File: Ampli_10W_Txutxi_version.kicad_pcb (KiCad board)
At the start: 2 copper layers, 35.3 x 31.7 mm, 9 parts, among them U1 TDA2003V

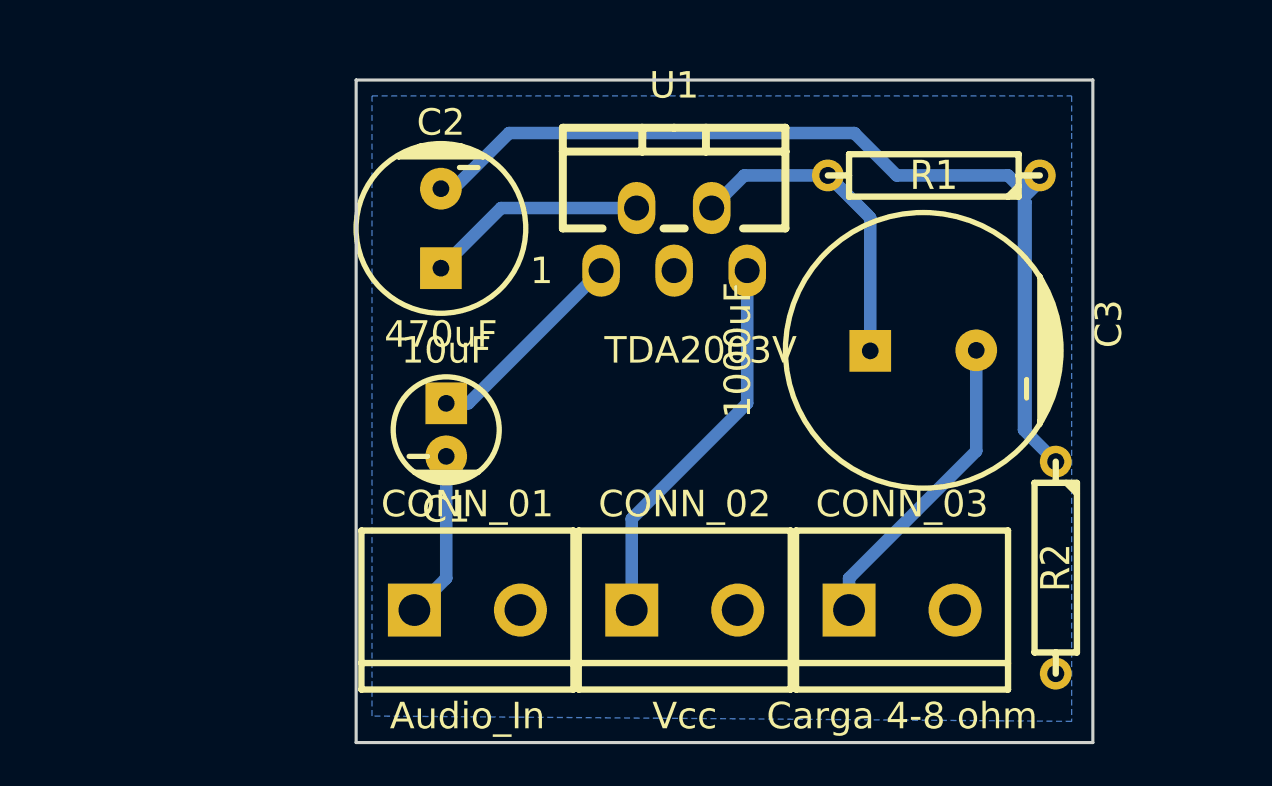
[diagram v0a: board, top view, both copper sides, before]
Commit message: Update library and PCB
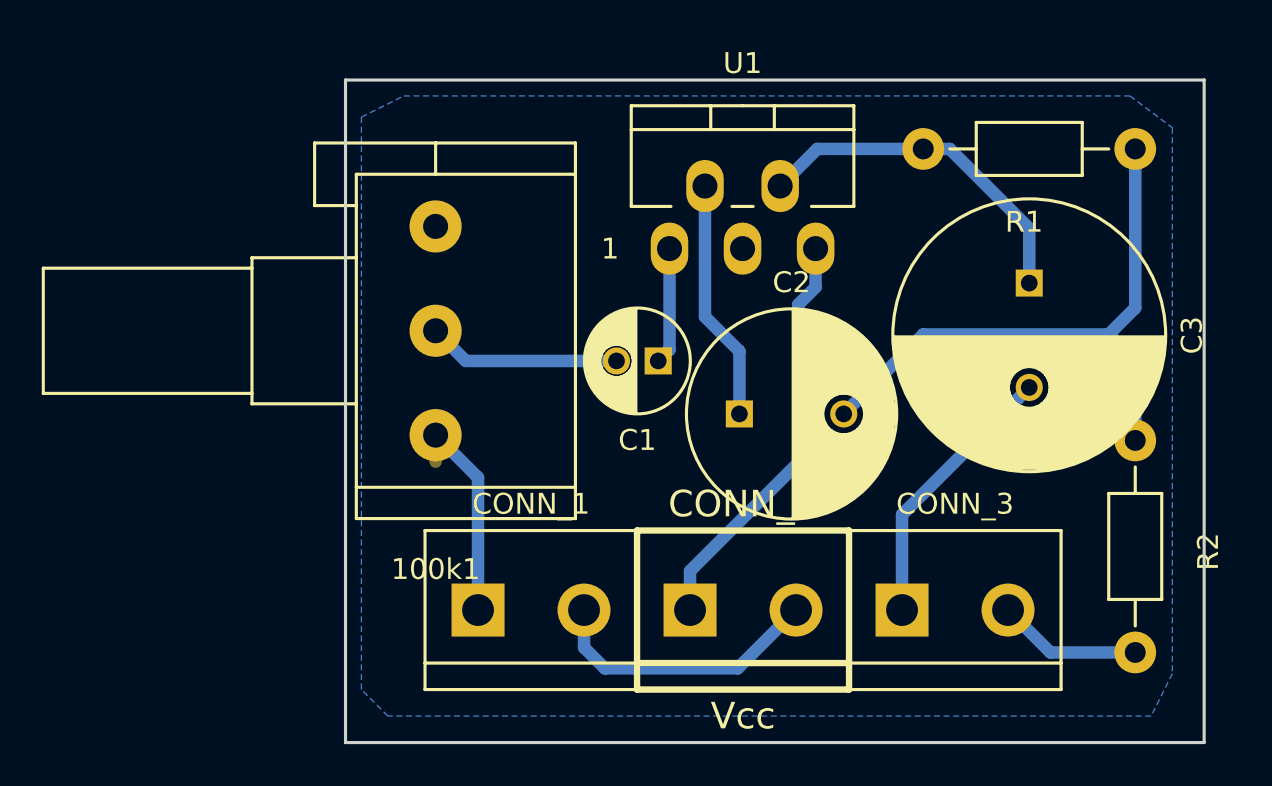
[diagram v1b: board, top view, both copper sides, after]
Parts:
- removed CONN_01: Audio_In, Connect:bornier2
- removed CONN_03: Carga 4-8 ohm, Connect:bornier2
- added 100k1: POT, Potentiometers:Potentiometer_Alps-RK16-single, F.Cu at (140.5, 114.0)
- added CONN_1: Audio_In, Connect:bornier2, F.Cu at (145.0, 122.4)
- added CONN_3: Carga 4-8 ohm, Connect:bornier2, F.Cu at (165.4, 122.4)
- C1: footprint Capacitors:CP_5x11mm -> Capacitors_ThroughHole:C_Radial_D5_L11_P2
- C2: footprint Capacitors:CP_8x21mm -> Capacitors_ThroughHole:C_Radial_D10_L16_P5
- C3: footprint Capacitors:CP_13x21mm -> Capacitors_ThroughHole:C_Radial_D13_L21_P5
- R1, R2: footprint Discret:R4 -> Resistors_ThroughHole:Resistor_Horizontal_RM10mm
- U1: footprint Pentawatts:Pentawatt_Neutral_Staggered_Verical_TO220-5-T05D -> TO_SOT_Packages_THT:Pentawatt_Neutral_Staggered_Verical_TO220-5-T05D
- moved C2 16.8 mm to (155.0, 113.0)
- moved C1 10.7 mm to (151.1, 110.5)
- moved R1 9.74 mm to (174.0, 100.3)
- moved R2 7.19 mm to (174.0, 114.3)
- moved C3 6.02 mm to (168.9, 106.8)
- moved U1 3.44 mm to (155.2, 101.3)
- moved CONN_2 2.79 mm to (155.2, 122.4)
- renumbered CONN_02 to CONN_2
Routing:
- net Net-(C2-Pad2): track 59.5 -> 29.3 mm
- net GND: track 0.00 -> 21.3 mm
- net +9V: track 30.8 -> 19.8 mm
- net Net-(100k1-Pad1): track 0.00 -> 10.5 mm
- net Net-(C3-Pad1): track 24.9 -> 17.3 mm
- net Net-(C1-Pad1): track 10.1 -> 5.61 mm
- net Net-(C3-Pad2): track 16.5 -> 13.2 mm
- net Net-(100k1-Pad2): track 8.00 -> 9.27 mm
- net Net-(C2-Pad1): track 10.6 -> 11.6 mm
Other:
- board size 35.3 x 31.7 mm -> 41.1 x 31.7 mm
